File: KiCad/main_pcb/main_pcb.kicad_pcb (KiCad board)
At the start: 2 copper layers, 69.7 x 75.1 mm, 57 parts, among them J1 Conn_01x06, J3 Conn_01x13, J4 Conn_01x07, J5 Conn_01x07, J6 USB_C_Receptacle_USB2.0_14P, J7 Conn_01x01, J8 Conn_01x01, SW1 SW_Push, U1 ATmega2560-16A, U2 TXB0104D, U3 TXB0104D, U4 TXB0104D, U5 CH340C, U6 AMS1117-3.3, Y1 Crystal_GND24

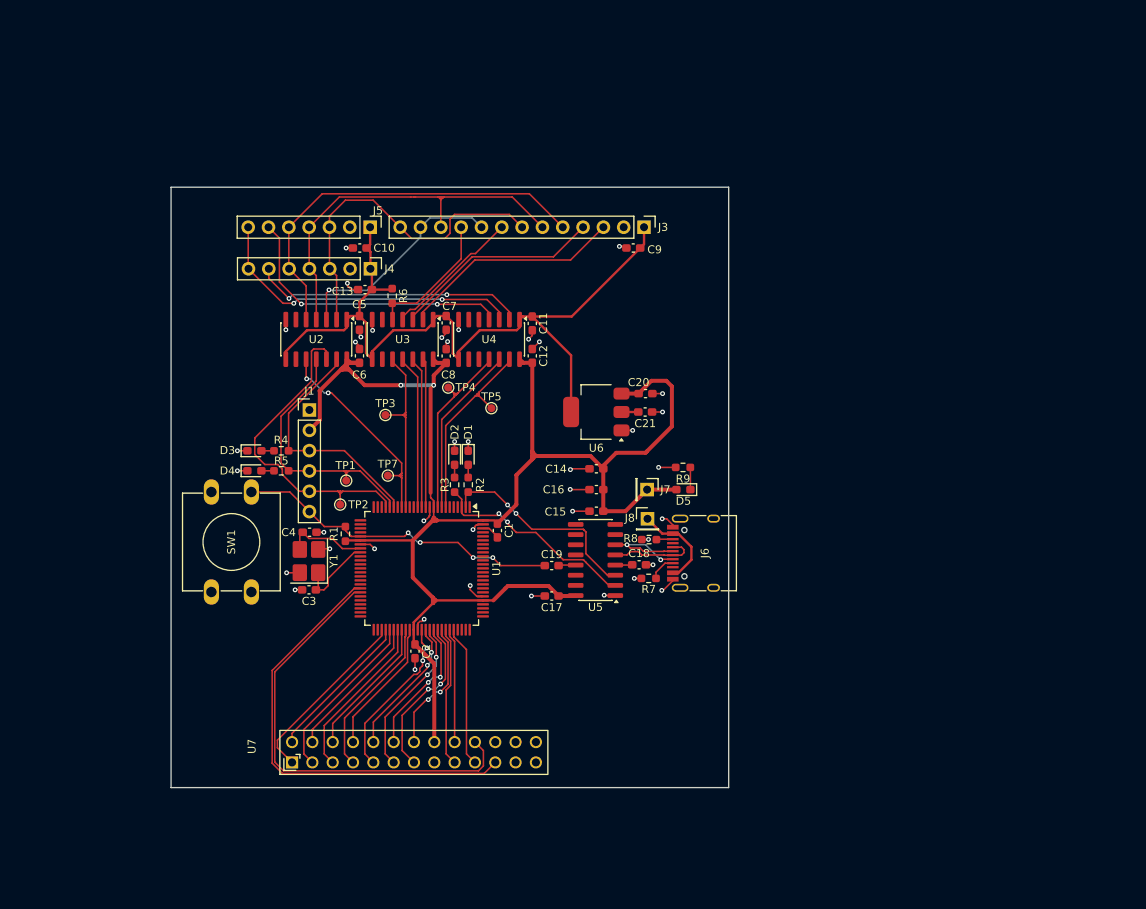
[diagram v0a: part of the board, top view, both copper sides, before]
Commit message: feat(pcb): Keeps working on version 2 of main PCB
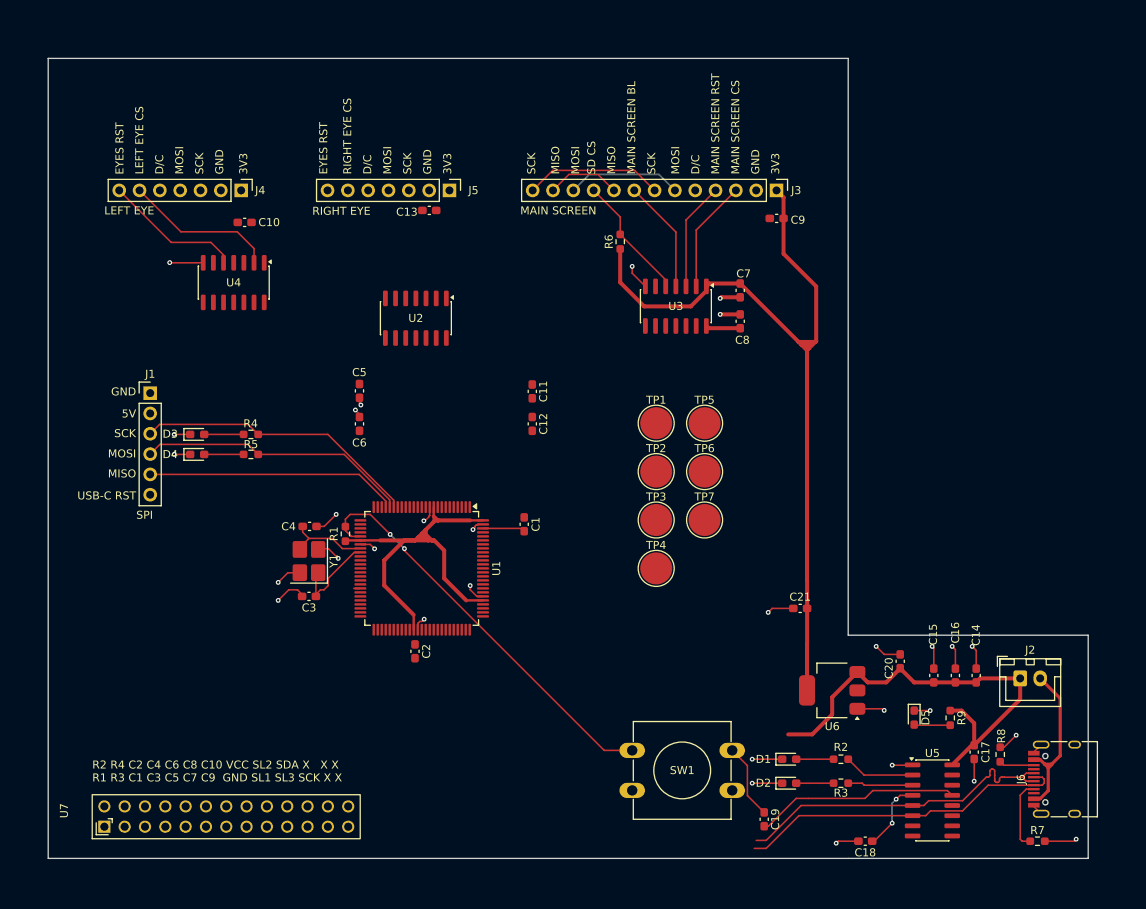
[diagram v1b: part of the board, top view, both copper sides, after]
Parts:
- removed J7, J8: Conn_01x01, Connector_PinHeader_2.54mm:PinHeader_1x01_P2.54mm_Vertical
- added J2: Conn_01x02, Connector_JST:JST_XH_B2B-XH-A_1x02_P2.50mm_Vertical, F.Cu at (164.5, 123.0)
- added TP6: Test Main Screen CS, TestPoint:TestPoint_Pad_D4.0mm, F.Cu at (125.0, 97.2)
- TP1, TP2, TP3, TP4, TP5, TP7: footprint TestPoint:TestPoint_Pad_D1.0mm -> TestPoint:TestPoint_Pad_D4.0mm
- moved R3 61.0 mm to (142.1, 136.1), turned to 180 degrees
- moved R7 58.7 mm to (166.7, 143.3), turned to 0 degrees
- moved D2 58.3 mm to (135.6, 136.1), turned to 0 degrees
- moved R2 57.9 mm to (142.1, 133.1), turned to 180 degrees
- moved SW1 57.5 mm to (116.0, 132.0), turned to 0 degrees
- moved C17 56.3 mm to (158.8, 132.2), turned to -90 degrees
- moved D1 55.0 mm to (135.6, 133.1), turned to 0 degrees
- moved C14 54.1 mm to (159.0, 122.6), turned to -90 degrees
- moved J6 53.2 mm to (170.2, 135.6)
- moved U5 51.7 mm to (153.5, 138.3), turned to 0 degrees
- moved R8 51.5 mm to (162.0, 132.5), turned to 90 degrees
- moved C16 50.5 mm to (156.4, 122.6), turned to -90 degrees
- moved C15 46.9 mm to (153.7, 122.6), turned to -90 degrees
- moved C20 46.2 mm to (149.5, 120.9), turned to -90 degrees
- moved R9 45.8 mm to (155.8, 127.9), turned to -90 degrees
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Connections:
- net Net-(J3-Pin_10) renamed /Screens/SD_CS-3V3
- net Net-(J3-Pin_3) renamed /Screens/MAIN_SCREEN_CS-3V3
- net Net-(J3-Pin_4) renamed /Screens/MAIN_SCREEN_RST-3V3
- net Net-(J3-Pin_5) renamed /Screens/DC-3V3
- net Net-(J3-Pin_8) renamed /Screens/MAIN_SCREEN_BL-3V3
- net Net-(J4-Pin_6) renamed /Screens/LEFT_EYE_CS-3V3
- net Net-(J5-Pin_6) renamed /Screens/RIGHT_EYE_CS-3V3
- D5 pad 1: Net-(D5-K) -> GND
- D5 pad 2: VCC -> Net-(D5-A)
- J4 pad 7: Net-(J4-Pin_7) -> /Screens/EYES_RST-3V3
- J5 pad 7: Net-(J4-Pin_7) -> /Screens/EYES_RST-3V3
- R9 pad 1: Net-(D5-K) -> VCC
- R9 pad 2: GND -> Net-(D5-A)
- U4 pad 10: unconnected-(U4-B4-Pad10) -> /Screens/Eyes_RST
- U4 pad 12: /Screens/Eyes_RST -> unconnected-(U4-B2-Pad12)
- U4 pad 3: Net-(J4-Pin_7) -> unconnected-(U4-A2-Pad3)
- U4 pad 5: unconnected-(U4-A4-Pad5) -> /Screens/EYES_RST-3V3
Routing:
- net VCC: track 192.3 -> 114.7 mm, vias 2 -> 0
- net /SDA: track 56.3 -> 0.00 mm
- net /SCL: track 56.7 -> 0.84 mm
- net /Screens/DC-3V3: track 50.1 -> 0.00 mm
- net Net-(J4-Pin_7): track 40.2 -> 0.00 mm, vias 2 -> 0
- net /Screens/RIGHT_EYE_CS-3V3: track 36.1 -> 0.00 mm, vias 2 -> 0
- net /Screens/MOSI_3V3: track 49.1 -> 14.4 mm
- net /USB-C/D+: track 11.0 -> 42.5 mm
- net GND: track 58.6 -> 86.2 mm, vias 40 -> 31
- net /USB-C/D-: track 14.1 -> 41.5 mm, vias 2 -> 0
- net /Screens/DC: track 26.8 -> 0.00 mm, vias 2 -> 0
- net /Screens/SCK_3V3: track 43.1 -> 17.3 mm
- net /Screens/Left_Eye_CS: track 25.3 -> 0.00 mm
- net Net-(U5-~{DTR}): track 2.16 -> 25.6 mm
- net /Screens/Right_Eye_CS: track 23.4 -> 0.00 mm
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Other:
- board size 69.7 x 75.1 mm -> 130 x 100 mm
- board text added: "3V3"
- board text added: "5V"
- board text added: "D/C"
- board text added: "EYES RST"
- board text added: "GND"
- board text added: "LEFT EYE"
- board text added: "LEFT EYE CS"
- board text added: "MAIN SCREEN"
- board text added: "MAIN SCREEN BL"
- board text added: "MAIN SCREEN CS"
- board text added: "MAIN SCREEN RST"
- board text added: "MISO"
- board text added: "MOSI"
- board text added: "R2 R4 C2 C4 C6 C8 C10 VCC SL2 SDA X X X R1 R3 C1 C3 C5 C7 C9 GND SL1 SL3 SCK X X"
- board text added: "RIGHT EYE"
- board text added: "RIGHT EYE CS"
- board text added: "SCK"
- board text added: "SD CS"
- board text added: "SPI"
- board text added: "USB-C RST"
